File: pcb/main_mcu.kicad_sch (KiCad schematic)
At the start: 31 parts, among them IC1 ATA6561-GAQW-N, J4 Screw_Terminal_01x03, U4 STM32H563VITx, Y1 25mHz 8pf, Y2 32.768kHz 12.5pF

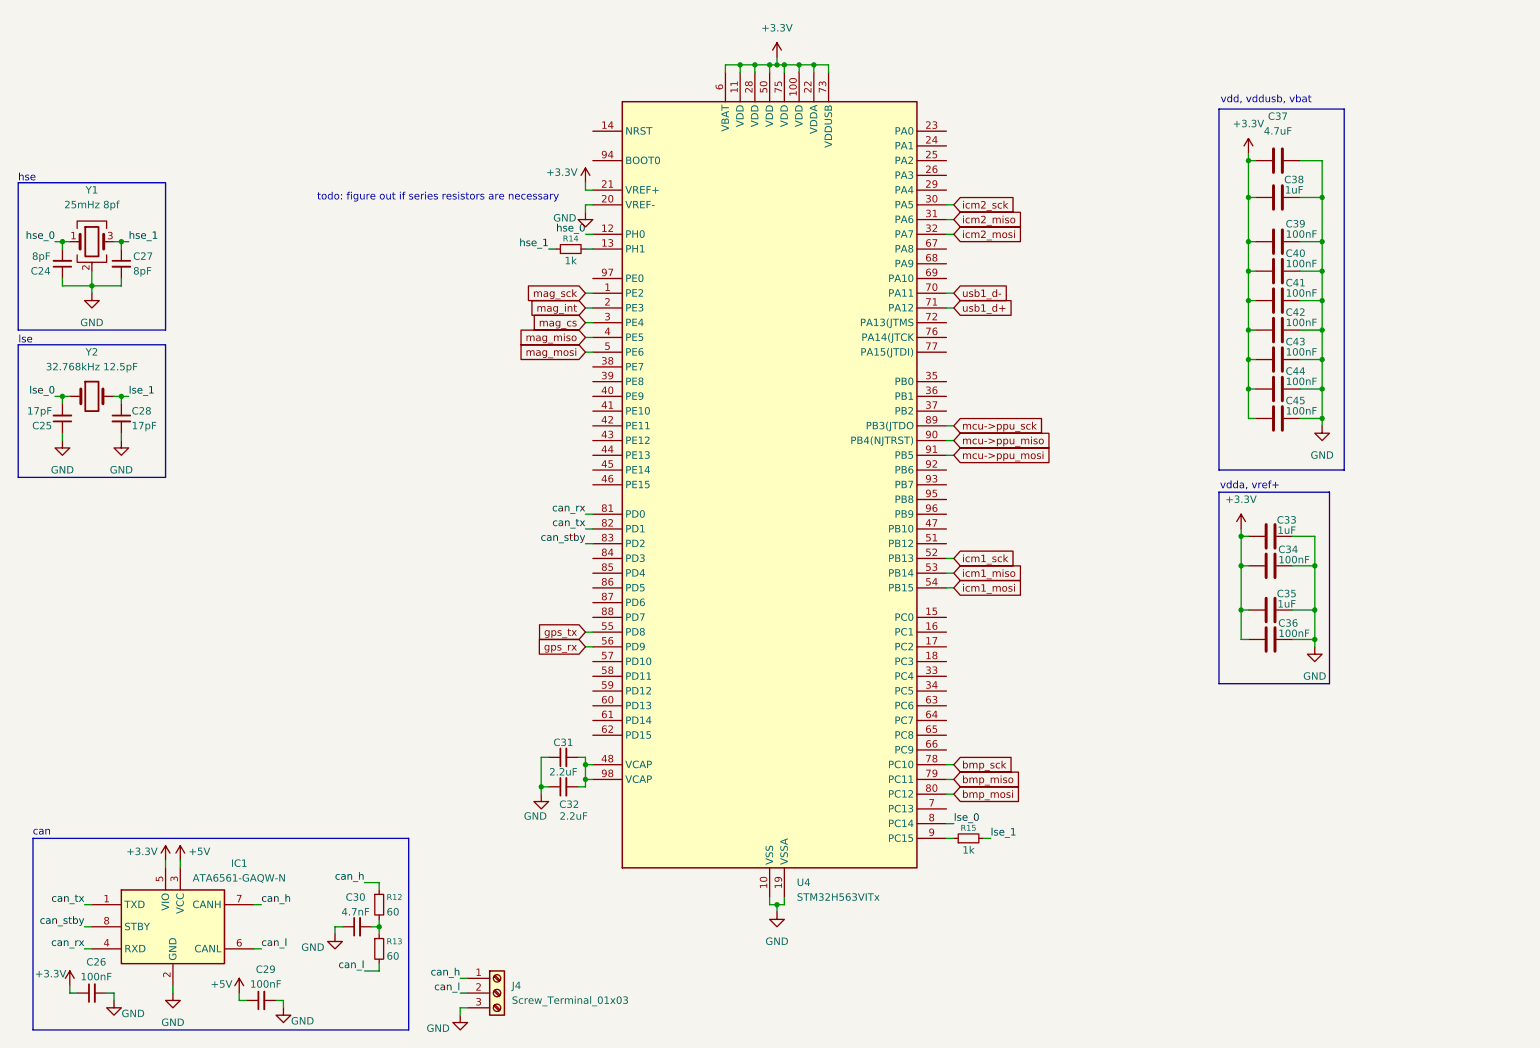
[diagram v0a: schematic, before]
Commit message: pretty much everything on schem done, though need to add circuit protection stuff and break out remaining pins
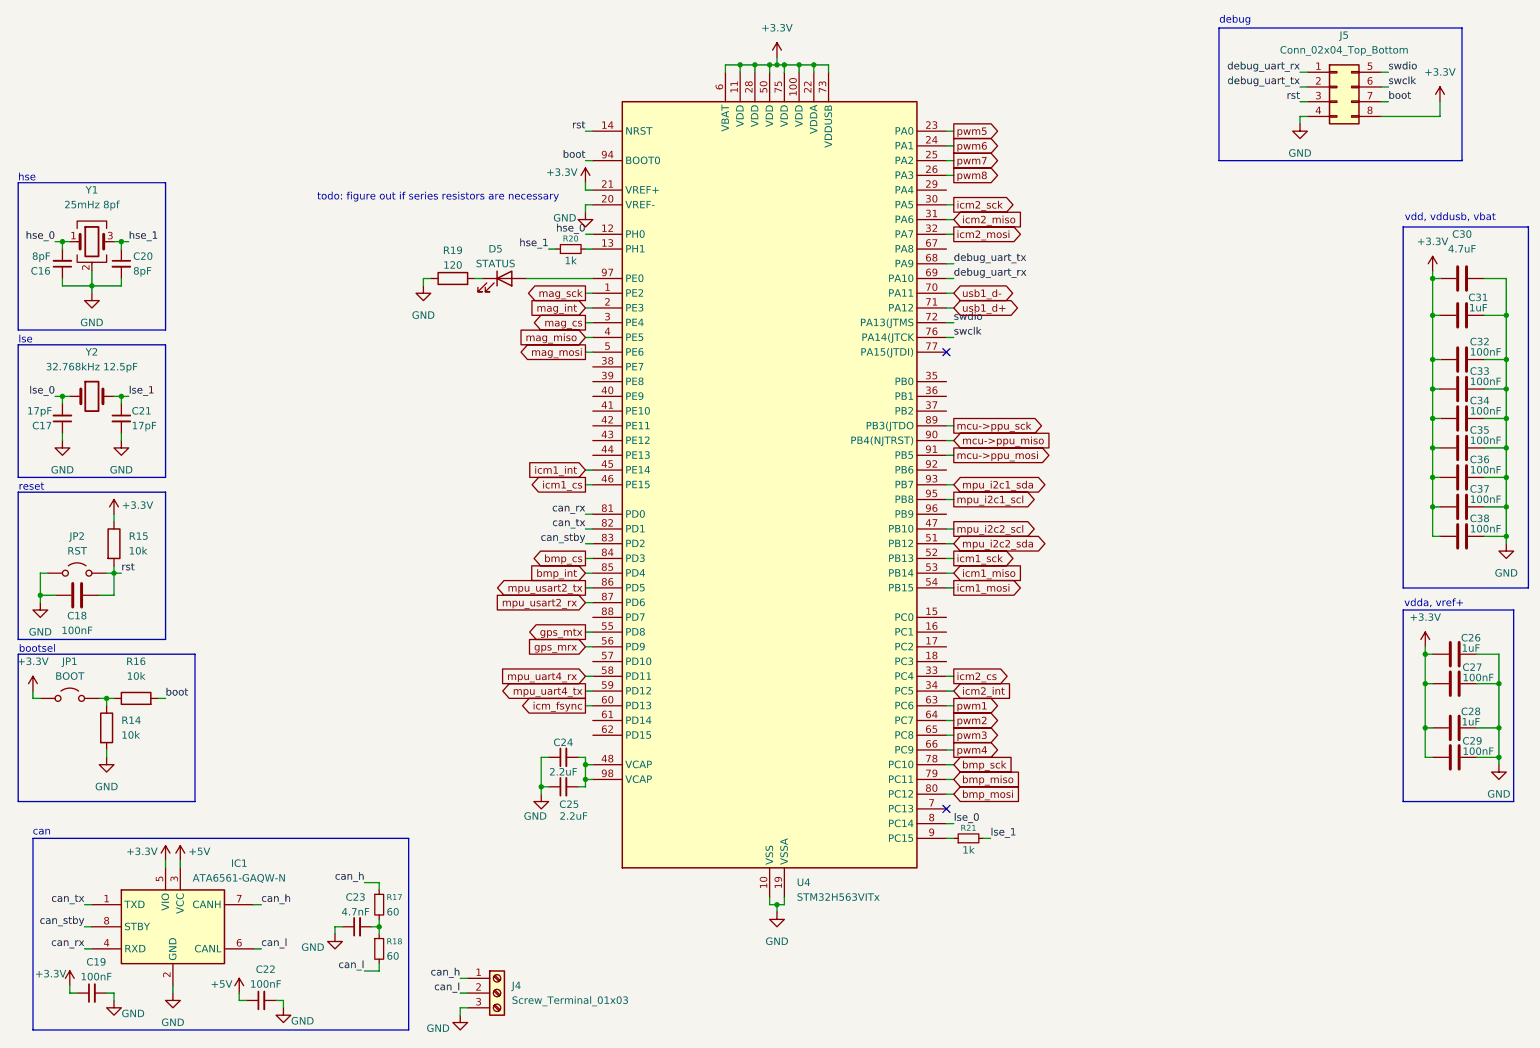
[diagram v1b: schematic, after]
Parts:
- added C18: 100nF, symbol Device:C
- added D5: STATUS, symbol Device:LED
- added J5: Conn_02x04_Top_Bottom, symbol Connector_Generic:Conn_02x04_Top_Bottom
- added JP1: BOOT, TestPoint:TestPoint_2Pads_Pitch2.54mm_Drill0.8mm, symbol Jumper:Jumper_2_Open
- added JP2: RST, TestPoint:TestPoint_2Pads_Pitch2.54mm_Drill0.8mm, symbol Jumper:Jumper_2_Open
- added R14, R15, R16: 10k, symbol Device:R
- added R19: 120, symbol Device:R
- renumbered C24 to C16, C25 to C17, C26 to C19, C27 to C20, C28 to C21, C29 to C22, C30 to C23, C31 to C24, C32 to C25, C33 to C26, C34 to C27, C35 to C28, C36 to C29, C37 to C30, C38 to C31, C39 to C32, C40 to C33, C41 to C34, C42 to C35, C43 to C36, C44 to C37, C45 to C38, R12 to R17, R13 to R18, R14 to R20, R15 to R21
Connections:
- net +3.3V: now also J5.8 (Pin_8), JP1.1 (A), R15.1
- net GND: now also C18.2, J5.4 (Pin_4), JP2.1 (A), R14.2, R19.1
- net rst: now reaches U4.14 (NRST)
- net rst: now also C18.1, J5.3 (Pin_3), JP2.2 (B), R15.2
- net pwm5: now reaches U4.23 (PA0)
- net pwm6: now reaches U4.24 (PA1)
- net pwm7: now reaches U4.25 (PA2)
- net pwm8: now reaches U4.26 (PA3)
- net icm2_cs: now reaches U4.33 (PC4)
- net icm2_int: now reaches U4.34 (PC5)
- net icm1_int: now reaches U4.45 (PE14)
- net icm1_cs: now reaches U4.46 (PE15)
- net mpu_i2c2_scl: now reaches U4.47 (PB10)
- net mpu_i2c2_sda: now reaches U4.51 (PB12)
- net mpu_uart4_rx: now reaches U4.58 (PD11)
- net mpu_uart4_tx: now reaches U4.59 (PD12)
- net icm_fsync: now reaches U4.60 (PD13)
- net pwm1: now reaches U4.63 (PC6)
- net pwm2: now reaches U4.64 (PC7)
- net pwm3: now reaches U4.65 (PC8)
- net pwm4: now reaches U4.66 (PC9)
- net debug_uart_tx: now reaches U4.68 (PA9)
- net debug_uart_tx: now also J5.2 (Pin_2)
- net debug_uart_rx: now reaches U4.69 (PA10)
- net debug_uart_rx: now also J5.1 (Pin_1)
- net swdio: now reaches U4.72 (PA13(JTMS)
- net swdio: now also J5.5 (Pin_5)
- net swclk: now reaches U4.76 (PA14(JTCK)
- net swclk: now also J5.6 (Pin_6)
- net bmp_cs: now reaches U4.84 (PD3)
- net bmp_int: now reaches U4.85 (PD4)
- net mpu_usart2_tx: now reaches U4.86 (PD5)
- net mpu_usart2_rx: now reaches U4.87 (PD6)
- net mpu_i2c1_sda: now reaches U4.93 (PB7)
- net boot: now reaches U4.94 (BOOT0)
- net boot: now also J5.7 (Pin_7), R16.2
- net mpu_i2c1_scl: now reaches U4.95 (PB8)
- net at U4.97 (PE0): now also D5.2 (A)
- net gps_rx renamed gps_mrx
- net gps_tx renamed gps_mtx
- new net: D5.1 (K), R19.2
- new net: JP1.2 (B), R14.1, R16.1
- no-connect marks 0 -> 2
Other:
- note added: "bootsel"
- note added: "debug"
- note added: "reset"
- moved on the sheet: C26, C27, C28, C29, C30, C31, C32, C33, C34, C35, C36, C37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
